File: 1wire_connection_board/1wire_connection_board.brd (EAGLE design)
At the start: 74.9 x 24.9 mm, 15 parts

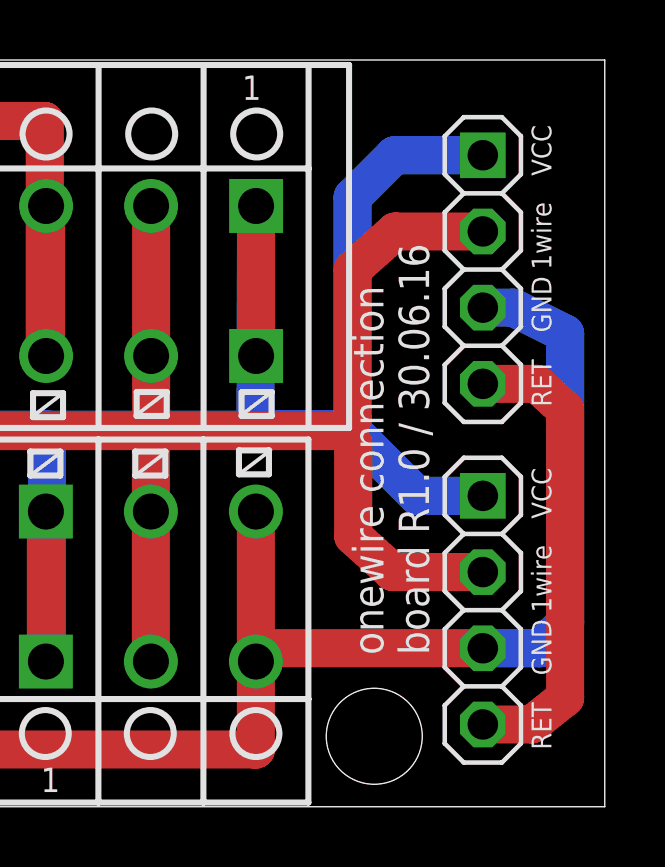
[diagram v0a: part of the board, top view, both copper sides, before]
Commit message: v1.1: Beschriftungen
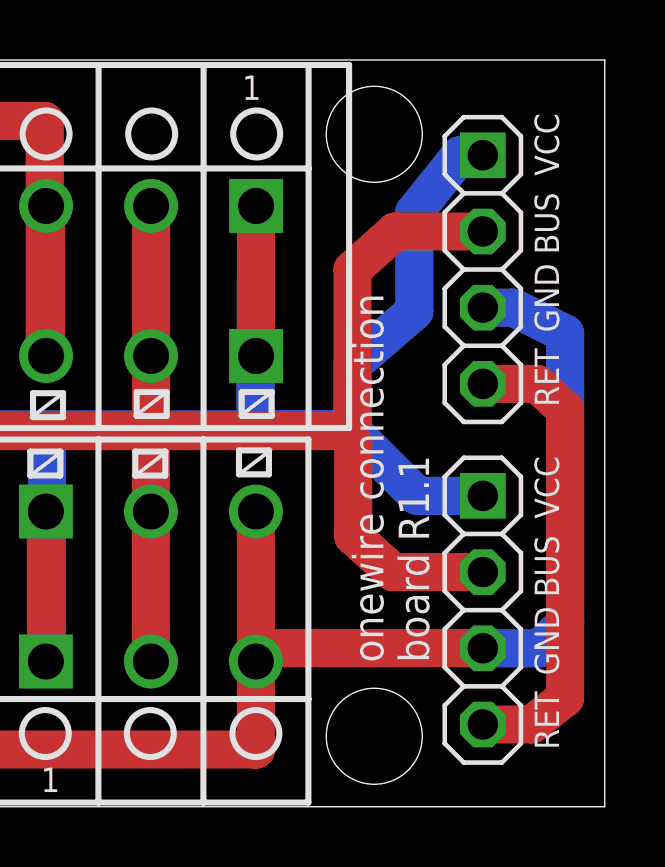
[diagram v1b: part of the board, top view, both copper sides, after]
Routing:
- net 1W_VCC: track 175.6 -> 174.3 mm
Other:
- board text added: "BUS"
- board text added: "onewire connection board R1.1"
- board text added: "onewire connection board R1.1 / 31.07.2016"
- board text removed: "1wire"
- board text removed: "onewire connection board R1.0 / 30.06.16"
